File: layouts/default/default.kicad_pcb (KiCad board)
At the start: 2 copper layers, 100 x 50 mm, 70 parts

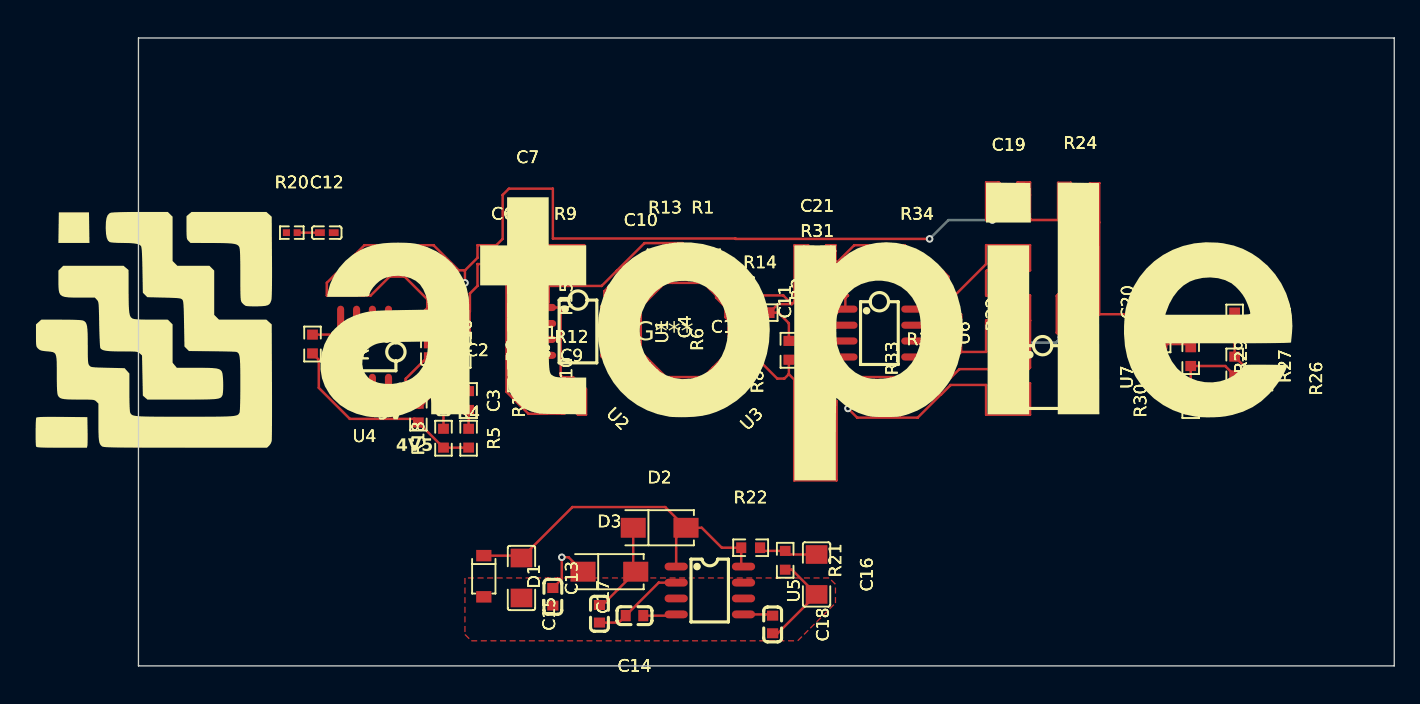
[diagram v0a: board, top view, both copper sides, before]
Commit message: layout updates
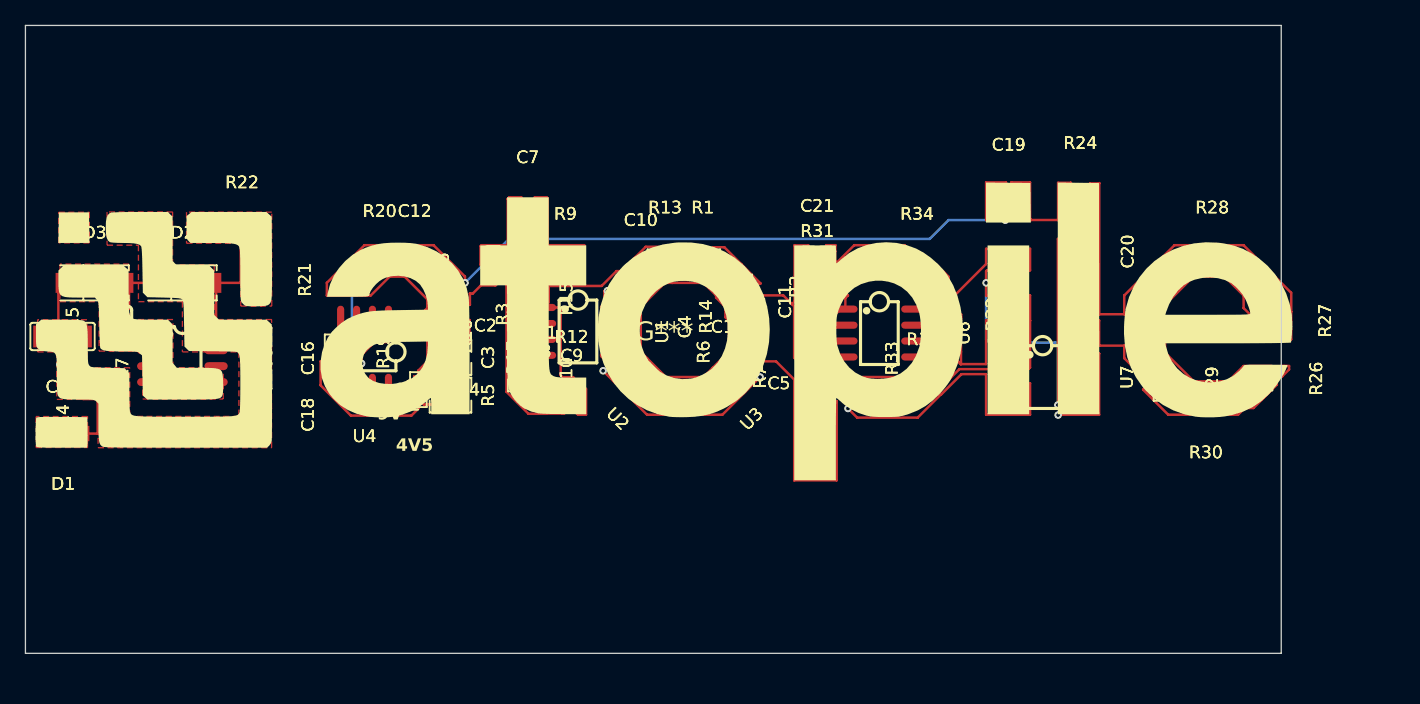
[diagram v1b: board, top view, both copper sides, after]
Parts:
- moved R21 47.8 mm to (84.2, 84.2)
- moved C16 47.7 mm to (84.5, 90.5)
- moved R22 47.6 mm to (83.2, 80.5)
- moved D3 47.0 mm to (71.5, 84.5)
- moved U5 45.9 mm to (78.5, 90.5)
- moved C15 44.4 mm to (73.8, 87.8)
- moved C14 44.3 mm to (73.0, 95.5), turned to 90 degrees
- moved C18 44.3 mm to (84.5, 95.0)
- moved D2 42.7 mm to (78.5, 84.5)
- moved C17 42.2 mm to (69.7, 91.8)
- moved C13 41.3 mm to (69.0, 88.8), turned to 180 degrees
- moved D1 35.4 mm to (69.0, 96.5), turned to 180 degrees
- moved C12 7.36 mm to (97.0, 82.8)
- moved R20 7.36 mm to (94.2, 82.8)
- moved R28 5.42 mm to (160.5, 82.5), turned to 0 degrees
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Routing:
- net INPUT: track 5.05 -> 37.8 mm
- net output_stage-gnd: track 5.81 -> 28.9 mm
- net output: track 15.6 -> 35.9 mm, vias 2 -> 3
- net hv-1: track 4.91 -> 18.3 mm, vias 1 -> 2
- net output_stage-net: track 0.00 -> 12.8 mm
- net input_stage-P1INplus: track 4.27 -> 15.2 mm, vias 0 -> 2
- net line: track 14.0 -> 24.8 mm
- net gnd-1: track 8.10 -> 18.1 mm, vias 0 -> 2
- net gain_stage-line: track 0.00 -> 8.44 mm
- net gain_stage-net-2: track 8.79 -> 15.9 mm
- net output-1: track 131.4 -> 126.7 mm
- net CAPplus: track 7.43 -> 3.49 mm
- net P1INminus: track 17.5 -> 20.3 mm
- net CAPminus: track 2.66 -> 0.00 mm
- net gnd-2: track 2.36 -> 0.00 mm
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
